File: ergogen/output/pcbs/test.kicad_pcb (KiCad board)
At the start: 2 copper layers, 20 x 20 mm, 1 part

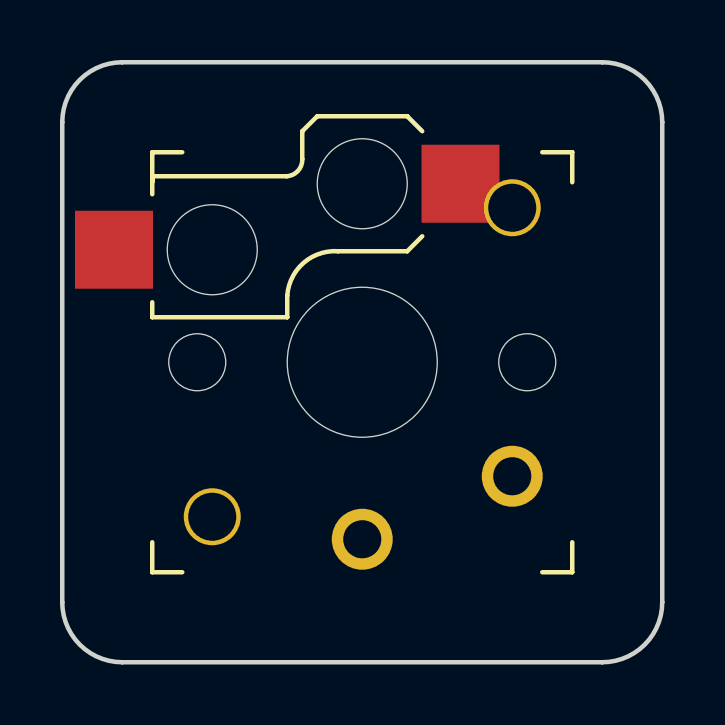
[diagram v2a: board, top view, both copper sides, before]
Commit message: update config
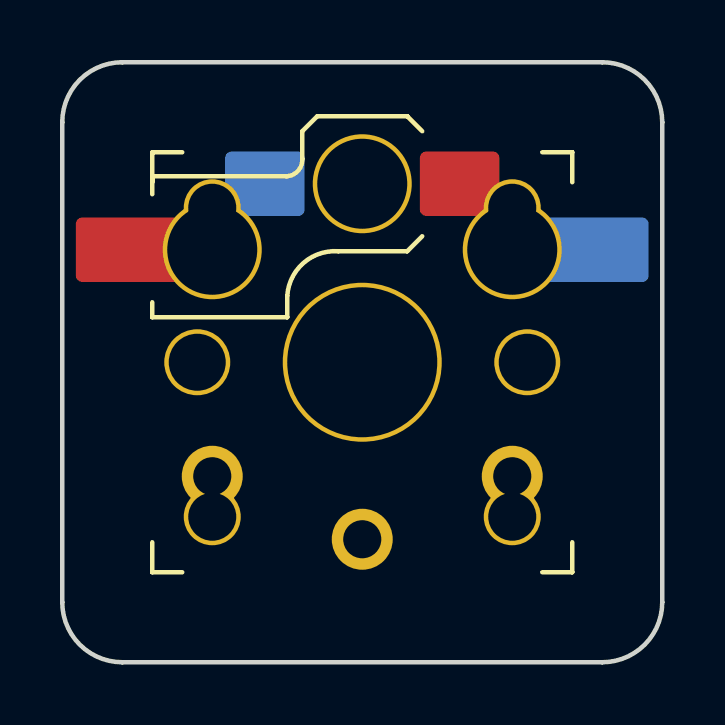
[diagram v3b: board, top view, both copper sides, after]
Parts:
- S1: moved to B.Cu
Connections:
- S1 pad : C3 -> middle_home
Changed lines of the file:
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@@
 (net 5 "D1")
     (footprint "ceoloide:switch_choc_v1_v2"
-      (layer "F.Cu")
+      (layer "B.Cu")
       (at 100 100 0)
       (property "Reference" "S1"
         (at 0 0 0)
-        (layer "F.SilkS")
+        (layer "B.SilkS")
         hide
-        (effects (font (size 1.27 1.27) (thickness 0.15)))
+        (effects (font (size 1 1) (thickness 0.15)))
       )
       (attr exclude_from_pos_files exclude_from_bom)
-    (pad "" np_thru_hole circle (at 0 0 0) (size 5 5) (drill 5) (layers "*.Cu" "*.Mask"))
-    (pad "" np_thru_hole circle (at 5.5 0 0) (size 1.9 1.9) (drill 1.9) (layers "*.Cu" "*.Mask"))
-    (pad "" np_thru_hole circle (at -5.5 0 0) (size 1.9 1.9) (drill 1.9) (layers "*.Cu" "*.Mask"))
+    (pad "" thru_hole circle (at 0 0 0) (size 5.3 5.3) (drill 5) (layers "*.Cu" "*.Mask") (net 3 "GND"))
+    (pad "" thru_hole circle (at 5.5 0 0) (size 2.1999999999999997 2.1999999999999997) (drill 1.9) (layers "*.Cu" "*.Mask"))
+    (pad "" thru_hole circle (at -5.5 0 0) (size 2.1999999999999997 2.1999999999999997) (drill 1.9) (layers "*.Cu" "*.Mask"))
     (fp_line (start -7 -6) (end -7 -7) (layer "F.SilkS") (stroke (width 0.15) (type solid)))
     (fp_line (start -7 7) (end -6 7) (layer "F.SilkS") (stroke (width 0.15) (type solid)))
@@
     (fp_line (start 6 7) (end 7 7) (layer "F.SilkS") (stroke (width 0.15) (type solid)))
     (fp_line (start 7 -7) (end 7 -6) (layer "F.SilkS") (stroke (width 0.15) (type solid)))
+    (fp_line (start -7 -6) (end -7 -7) (layer "B.SilkS") (stroke (width 0.15) (type solid)))
+    (fp_line (start -7 7) (end -6 7) (layer "B.SilkS") (stroke (width 0.15) (type solid)))
+    (fp_line (start -6 -7) (end -7 -7) (layer "B.SilkS") (stroke (width 0.15) (type solid)))
+    (fp_line (start -7 7) (end -7 6) (layer "B.SilkS") (stroke (width 0.15) (type solid)))
+    (fp_line (start 7 6) (end 7 7) (layer "B.SilkS") (stroke (width 0.15) (type solid)))
+    (fp_line (start 7 -7) (end 6 -7) (layer "B.SilkS") (stroke (width 0.15) (type solid)))
+    (fp_line (start 6 7) (end 7 7) (layer "B.SilkS") (stroke (width 0.15) (type solid)))
+    (fp_line (start 7 -7) (end 7 -6) (layer "B.SilkS") (stroke (width 0.15) (type solid)))
     (fp_line (start -8.75 -8.25) (end 8.75 -8.25) (layer "Dwgs.User") (stroke (width 0.15) (type solid)))
     (fp_line (start 8.75 -8.25) (end 8.75 8.25) (layer "Dwgs.User") (stroke (width 0.15) (type solid)))
@@
     (fp_line (start -8.75 8.25) (end -8.75 -8.25) (layer "Dwgs.User") (stroke (width 0.15) (type solid)))
     (pad "" thru_hole circle (at -5.00 5.15 0) (size 1.9 1.9) (drill 1.6) (layers "*.Cu" "*.Mask") (net 2 "middle_home"))
-    (pad "" thru_hole circle (at 5.00 -5.15 0) (size 1.9 1.9) (drill 1.6) (layers "*.Cu" "*.Mask") (net 1 "C3"))
-    (pad "" np_thru_hole circle (at 0 -5.95 0) (size 3 3) (drill 3) (layers "*.Cu" "*.Mask"))
+    (pad "" thru_hole circle (at 5.00 -5.15 0) (size 1.9 1.9) (drill 1.6) (layers "*.Cu" "*.Mask") (net 2 "middle_home"))
+    (pad "" thru_hole circle (at 5.00 5.15 0) (size 1.9 1.9) (drill 1.6) (layers "*.Cu" "*.Mask") (net 2 "middle_home"))
+    (pad "" thru_hole circle (at -5.00 -5.15 0) (size 1.9 1.9) (drill 1.6) (layers "*.Cu" "*.Mask") (net 1 "C3"))
+    (pad "" thru_hole circle (at 0 -5.95 0) (size 3.3 3.3) (drill 3) (layers "*.Cu" "*.Mask") )
     (fp_line (start -7 -5.6) (end -7 -6.2) (layer "F.SilkS") (stroke (width 0.15) (type solid)))
     (fp_line (start -7 -6.2) (end -2.52 -6.2) (layer "F.SilkS") (stroke (width 0.15) (type solid)))
@@
     (fp_line (start 2 -4.2) (end 1.5 -3.7) (layer "F.SilkS") (stroke (width 0.15) (type solid)))
     (fp_arc (start -2.5 -2.22) (mid -1.956518 -3.312082) (end -0.8 -3.7) (layer "F.SilkS") (stroke (width 0.15) (type solid)))
-    (pad "" np_thru_hole circle (at -5 -3.75 195) (size 3 3) (drill 3) (layers "*.Cu" "*.Mask"))
-    (pad "1" smd rect (at 3.275 -5.95 0) (size 2.6 2.6) (layers "F.Cu" "F.Paste" "F.Mask") (net 1 "C3"))
-    (pad "2" smd rect (at -8.275 -3.75 0) (size 2.6 2.6) (layers "F.Cu" "F.Paste" "F.Mask") (net 2 "middle_home"))
+    (pad "1" thru_hole circle (at -5 -3.75 195) (size 3.3 3.3) (drill 3) (layers "*.Cu" "*.Mask") (net 1 "C3"))
+    (pad "2" smd roundrect (at 3.245 -5.95 0) (size 2.65 2.15) (layers "F.Cu" "F.Paste" "F.Mask") (roundrect_rratio 0.1) (net 2 "middle_home"))
+    (pad "1" smd roundrect (at -7.6475 -3.75 0) (size 3.8 2.15) (layers "F.Cu") (roundrect_rratio 0.1) (net 1 "C3"))
+    (pad "" smd roundrect (at -8.2475 -3.75 0) (size 2.6 2.15) (layers "F.Paste" "F.Mask") (roundrect_rratio 0.1) (net 1 "C3"))
+    (fp_line (start -1.5 -8.2) (end -2 -7.7) (layer "B.SilkS") (stroke (width 0.15) (type solid)))
+    (fp_line (start 1.5 -8.2) (end -1.5 -8.2) (layer "B.SilkS") (stroke (width 0.15) (type solid)))
+    (fp_line (start 2 -7.7) (end 1.5 -8.2) (layer "B.SilkS") (stroke (width 0.15) (type solid)))
+    (fp_line (start 2 -7.7) (end 2 -6.78) (layer "B.SilkS") (stroke (width 0.15) (type solid)))
+    (fp_line (start 2.52 -6.2) (end 7 -6.2) (layer "B.SilkS") (stroke (width 0.15) (type solid)))
+    (fp_line (start 7 -6.2) (end 7 -5.6) (layer "B.SilkS") (stroke (width 0.15) (type solid)))
+    (fp_arc (start 2.52 -6.2) (mid 2.139878 -6.382304) (end 2 -6.78) (layer "B.SilkS") (stroke (width 0.15) (type solid)))
+    (fp_line (start -1.5 -3.7) (end -2 -4.2) (layer "B.SilkS") (stroke (width 0.15) (type solid)))
+    (fp_line (start 0.8 -3.7) (end -1.5 -3.7) (layer "B.SilkS") (stroke (width 0.15) (type solid)))
+    (fp_line (start 2.5 -1.5) (end 2.5 -2.2) (layer "B.SilkS") (stroke (width 0.15) (type solid)))
+    (fp_line (start 7 -1.5) (end 2.5 -1.5) (layer "B.SilkS") (stroke (width 0.15) (type solid)))
+    (fp_line (start 7 -2) (end 7 -1.5) (layer "B.SilkS") (stroke (width 0.15) (type solid)))
+    (fp_arc (start 0.8 -3.7) (mid 1.956518 -3.312082) (end 2.5 -2.22) (layer "B.SilkS") (stroke (width 0.15) (type solid)))
+      (pad "2" thru_hole circle (at 5 -3.75 195) (size 3.3 3.3) (drill 3) (layers "*.Cu" "*.Mask") (net 2 "middle_home"))
+    (pad "1" smd roundrect (at -3.245 -5.95 0) (size 2.65 2.15) (layers "B.Cu" "B.Paste" "B.Mask") (roundrect_rratio 0.1) (net 1 "C3"))
+    (pad "2" smd roundrect (at 7.6475 -3.75 0) (size 3.8 2.15) (layers "B.Cu") (roundrect_rratio 0.1) (net 2 "middle_home"))
+    (pad "" smd roundrect (at 8.2475 -3.75 0) (size 2.6 2.15) (layers "B.Paste" "B.Mask") (roundrect_rratio 0.1) (net 2 "middle_home"))
     (pad "2" thru_hole circle (at 0 5.9 195) (size 2.032 2.032) (drill 1.27) (layers "*.Cu" "*.Mask") (net 1 "C3"))
     (pad "1" thru_hole circle (at 5 3.8 195) (size 2.032 2.032) (drill 1.27) (layers "*.Cu" "*.Mask") (net 2 "middle_home"))
+    (pad "1" thru_hole circle (at -5 3.8 195) (size 2.032 2.032) (drill 1.27) (layers "*.Cu" "*.Mask") (net 2 "middle_home"))
   )
   (gr_line (start 92 110) (end 108 110) (layer Edge.Cuts) (stroke (width 0.15) (type default)))

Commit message: changes
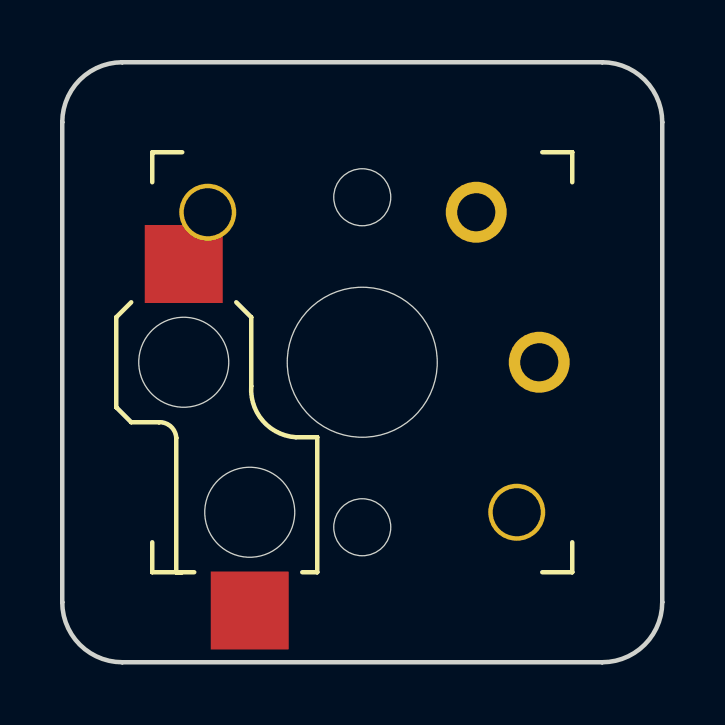
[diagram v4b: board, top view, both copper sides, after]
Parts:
- S1: moved to F.Cu
- turned S1 to 90 degrees
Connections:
- S1 pad : middle_home -> C3
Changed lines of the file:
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@@
   (title_block
     (title "test")
-    (date "2024-04-21")
+    (date "2024-04-22")
     (rev "0.1")
     (company "nxtk")
@@
 (net 2 "middle_home")
 (net 3 "GND")
-(net 4 "D2")
-(net 5 "D1")
+(net 4 "D1")
+(net 5 "D2")
     (footprint "ceoloide:switch_choc_v1_v2"
-      (layer "B.Cu")
-      (at 100 100 0)
+      (layer "F.Cu")
+      (at 100 100 90)
       (property "Reference" "S1"
-        (at 0 0 0)
-        (layer "B.SilkS")
+        (at 0 0 90)
+        (layer "F.SilkS")
         hide
         (effects (font (size 1 1) (thickness 0.15)))
       )
       (attr exclude_from_pos_files exclude_from_bom)
-    (pad "" thru_hole circle (at 0 0 0) (size 5.3 5.3) (drill 5) (layers "*.Cu" "*.Mask") (net 3 "GND"))
-    (pad "" thru_hole circle (at 5.5 0 0) (size 2.1999999999999997 2.1999999999999997) (drill 1.9) (layers "*.Cu" "*.Mask"))
-    (pad "" thru_hole circle (at -5.5 0 0) (size 2.1999999999999997 2.1999999999999997) (drill 1.9) (layers "*.Cu" "*.Mask"))
+    (pad "" np_thru_hole circle (at 0 0 90) (size 5 5) (drill 5) (layers "*.Cu" "*.Mask"))
+    (pad "" np_thru_hole circle (at 5.5 0 90) (size 1.9 1.9) (drill 1.9) (layers "*.Cu" "*.Mask"))
+    (pad "" np_thru_hole circle (at -5.5 0 90) (size 1.9 1.9) (drill 1.9) (layers "*.Cu" "*.Mask"))
     (fp_line (start -7 -6) (end -7 -7) (layer "F.SilkS") (stroke (width 0.15) (type solid)))
     (fp_line (start -7 7) (end -6 7) (layer "F.SilkS") (stroke (width 0.15) (type solid)))
@@
     (fp_line (start 6 7) (end 7 7) (layer "F.SilkS") (stroke (width 0.15) (type solid)))
     (fp_line (start 7 -7) (end 7 -6) (layer "F.SilkS") (stroke (width 0.15) (type solid)))
-    (fp_line (start -7 -6) (end -7 -7) (layer "B.SilkS") (stroke (width 0.15) (type solid)))
-    (fp_line (start -7 7) (end -6 7) (layer "B.SilkS") (stroke (width 0.15) (type solid)))
-    (fp_line (start -6 -7) (end -7 -7) (layer "B.SilkS") (stroke (width 0.15) (type solid)))
-    (fp_line (start -7 7) (end -7 6) (layer "B.SilkS") (stroke (width 0.15) (type solid)))
-    (fp_line (start 7 6) (end 7 7) (layer "B.SilkS") (stroke (width 0.15) (type solid)))
-    (fp_line (start 7 -7) (end 6 -7) (layer "B.SilkS") (stroke (width 0.15) (type solid)))
-    (fp_line (start 6 7) (end 7 7) (layer "B.SilkS") (stroke (width 0.15) (type solid)))
-    (fp_line (start 7 -7) (end 7 -6) (layer "B.SilkS") (stroke (width 0.15) (type solid)))
     (fp_line (start -8.75 -8.25) (end 8.75 -8.25) (layer "Dwgs.User") (stroke (width 0.15) (type solid)))
     (fp_line (start 8.75 -8.25) (end 8.75 8.25) (layer "Dwgs.User") (stroke (width 0.15) (type solid)))
     (fp_line (start 8.75 8.25) (end -8.75 8.25) (layer "Dwgs.User") (stroke (width 0.15) (type solid)))
     (fp_line (start -8.75 8.25) (end -8.75 -8.25) (layer "Dwgs.User") (stroke (width 0.15) (type solid)))
-    (pad "" thru_hole circle (at -5.00 5.15 0) (size 1.9 1.9) (drill 1.6) (layers "*.Cu" "*.Mask") (net 2 "middle_home"))
-    (pad "" thru_hole circle (at 5.00 -5.15 0) (size 1.9 1.9) (drill 1.6) (layers "*.Cu" "*.Mask") (net 2 "middle_home"))
-    (pad "" thru_hole circle (at 5.00 5.15 0) (size 1.9 1.9) (drill 1.6) (layers "*.Cu" "*.Mask") (net 2 "middle_home"))
-    (pad "" thru_hole circle (at -5.00 -5.15 0) (size 1.9 1.9) (drill 1.6) (layers "*.Cu" "*.Mask") (net 1 "C3"))
-    (pad "" thru_hole circle (at 0 -5.95 0) (size 3.3 3.3) (drill 3) (layers "*.Cu" "*.Mask") )
+    (pad "" thru_hole circle (at -5.00 5.15 90) (size 1.9 1.9) (drill 1.6) (layers "*.Cu" "*.Mask") (net 2 "middle_home"))
+    (pad "" thru_hole circle (at 5.00 -5.15 90) (size 1.9 1.9) (drill 1.6) (layers "*.Cu" "*.Mask") (net 1 "C3"))
+    (pad "" np_thru_hole circle (at 0 -5.95 90) (size 3 3) (drill 3) (layers "*.Cu" "*.Mask"))
     (fp_line (start -7 -5.6) (end -7 -6.2) (layer "F.SilkS") (stroke (width 0.15) (type solid)))
     (fp_line (start -7 -6.2) (end -2.52 -6.2) (layer "F.SilkS") (stroke (width 0.15) (type solid)))
@@
     (fp_line (start 2 -4.2) (end 1.5 -3.7) (layer "F.SilkS") (stroke (width 0.15) (type solid)))
     (fp_arc (start -2.5 -2.22) (mid -1.956518 -3.312082) (end -0.8 -3.7) (layer "F.SilkS") (stroke (width 0.15) (type solid)))
-    (pad "1" thru_hole circle (at -5 -3.75 195) (size 3.3 3.3) (drill 3) (layers "*.Cu" "*.Mask") (net 1 "C3"))
-    (pad "2" smd roundrect (at 3.245 -5.95 0) (size 2.65 2.15) (layers "F.Cu" "F.Paste" "F.Mask") (roundrect_rratio 0.1) (net 2 "middle_home"))
-    (pad "1" smd roundrect (at -7.6475 -3.75 0) (size 3.8 2.15) (layers "F.Cu") (roundrect_rratio 0.1) (net 1 "C3"))
-    (pad "" smd roundrect (at -8.2475 -3.75 0) (size 2.6 2.15) (layers "F.Paste" "F.Mask") (roundrect_rratio 0.1) (net 1 "C3"))
-    (fp_line (start -1.5 -8.2) (end -2 -7.7) (layer "B.SilkS") (stroke (width 0.15) (type solid)))
-    (fp_line (start 1.5 -8.2) (end -1.5 -8.2) (layer "B.SilkS") (stroke (width 0.15) (type solid)))
-    (fp_line (start 2 -7.7) (end 1.5 -8.2) (layer "B.SilkS") (stroke (width 0.15) (type solid)))
-    (fp_line (start 2 -7.7) (end 2 -6.78) (layer "B.SilkS") (stroke (width 0.15) (type solid)))
-    (fp_line (start 2.52 -6.2) (end 7 -6.2) (layer "B.SilkS") (stroke (width 0.15) (type solid)))
-    (fp_line (start 7 -6.2) (end 7 -5.6) (layer "B.SilkS") (stroke (width 0.15) (type solid)))
-    (fp_arc (start 2.52 -6.2) (mid 2.139878 -6.382304) (end 2 -6.78) (layer "B.SilkS") (stroke (width 0.15) (type solid)))
-    (fp_line (start -1.5 -3.7) (end -2 -4.2) (layer "B.SilkS") (stroke (width 0.15) (type solid)))
-    (fp_line (start 0.8 -3.7) (end -1.5 -3.7) (layer "B.SilkS") (stroke (width 0.15) (type solid)))
-    (fp_line (start 2.5 -1.5) (end 2.5 -2.2) (layer "B.SilkS") (stroke (width 0.15) (type solid)))
-    (fp_line (start 7 -1.5) (end 2.5 -1.5) (layer "B.SilkS") (stroke (width 0.15) (type solid)))
-    (fp_line (start 7 -2) (end 7 -1.5) (layer "B.SilkS") (stroke (width 0.15) (type solid)))
-    (fp_arc (start 0.8 -3.7) (mid 1.956518 -3.312082) (end 2.5 -2.22) (layer "B.SilkS") (stroke (width 0.15) (type solid)))
-      (pad "2" thru_hole circle (at 5 -3.75 195) (size 3.3 3.3) (drill 3) (layers "*.Cu" "*.Mask") (net 2 "middle_home"))
-    (pad "1" smd roundrect (at -3.245 -5.95 0) (size 2.65 2.15) (layers "B.Cu" "B.Paste" "B.Mask") (roundrect_rratio 0.1) (net 1 "C3"))
-    (pad "2" smd roundrect (at 7.6475 -3.75 0) (size 3.8 2.15) (layers "B.Cu") (roundrect_rratio 0.1) (net 2 "middle_home"))
-    (pad "" smd roundrect (at 8.2475 -3.75 0) (size 2.6 2.15) (layers "B.Paste" "B.Mask") (roundrect_rratio 0.1) (net 2 "middle_home"))
-    (pad "2" thru_hole circle (at 0 5.9 195) (size 2.032 2.032) (drill 1.27) (layers "*.Cu" "*.Mask") (net 1 "C3"))
-    (pad "1" thru_hole circle (at 5 3.8 195) (size 2.032 2.032) (drill 1.27) (layers "*.Cu" "*.Mask") (net 2 "middle_home"))
-    (pad "1" thru_hole circle (at -5 3.8 195) (size 2.032 2.032) (drill 1.27) (layers "*.Cu" "*.Mask") (net 2 "middle_home"))
+    (pad "" np_thru_hole circle (at -5 -3.75 285) (size 3 3) (drill 3) (layers "*.Cu" "*.Mask"))
+    (pad "1" smd rect (at 3.275 -5.95 90) (size 2.6 2.6) (layers "F.Cu" "F.Paste" "F.Mask") (net 1 "C3"))
+    (pad "2" smd rect (at -8.275 -3.75 90) (size 2.6 2.6) (layers "F.Cu" "F.Paste" "F.Mask") (net 2 "middle_home"))
+    (pad "2" thru_hole circle (at 0 5.9 285) (size 2.032 2.032) (drill 1.27) (layers "*.Cu" "*.Mask") (net 1 "C3"))
+    (pad "1" thru_hole circle (at 5 3.8 285) (size 2.032 2.032) (drill 1.27) (layers "*.Cu" "*.Mask") (net 2 "middle_home"))
   )
   (gr_line (start 92 110) (end 108 110) (layer Edge.Cuts) (stroke (width 0.15) (type default)))
